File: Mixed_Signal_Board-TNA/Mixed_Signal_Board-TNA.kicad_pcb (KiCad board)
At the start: 4 copper layers, 109 parts, among them J200 USB_C_Receptacle_USB2.0_14P, J201 2x5 1.27mm, J300 031-5640-1010, J400 031-5640-1010, U100 HT7533, U102 TLV62569DBV, U2 MCP6001T-E/OT, U200 STM32F103CBT6, U201 USBLC6-2SC6, U300 MCP6001T-E/OT, U301 MCP6001T-E/OT, U302 REF3033AIDBZT, U303 ADC141S626CIMM_NOPB, U304 MCP6001T-E/OT, U400 DAC7563SDGSR, Y200 16MHz

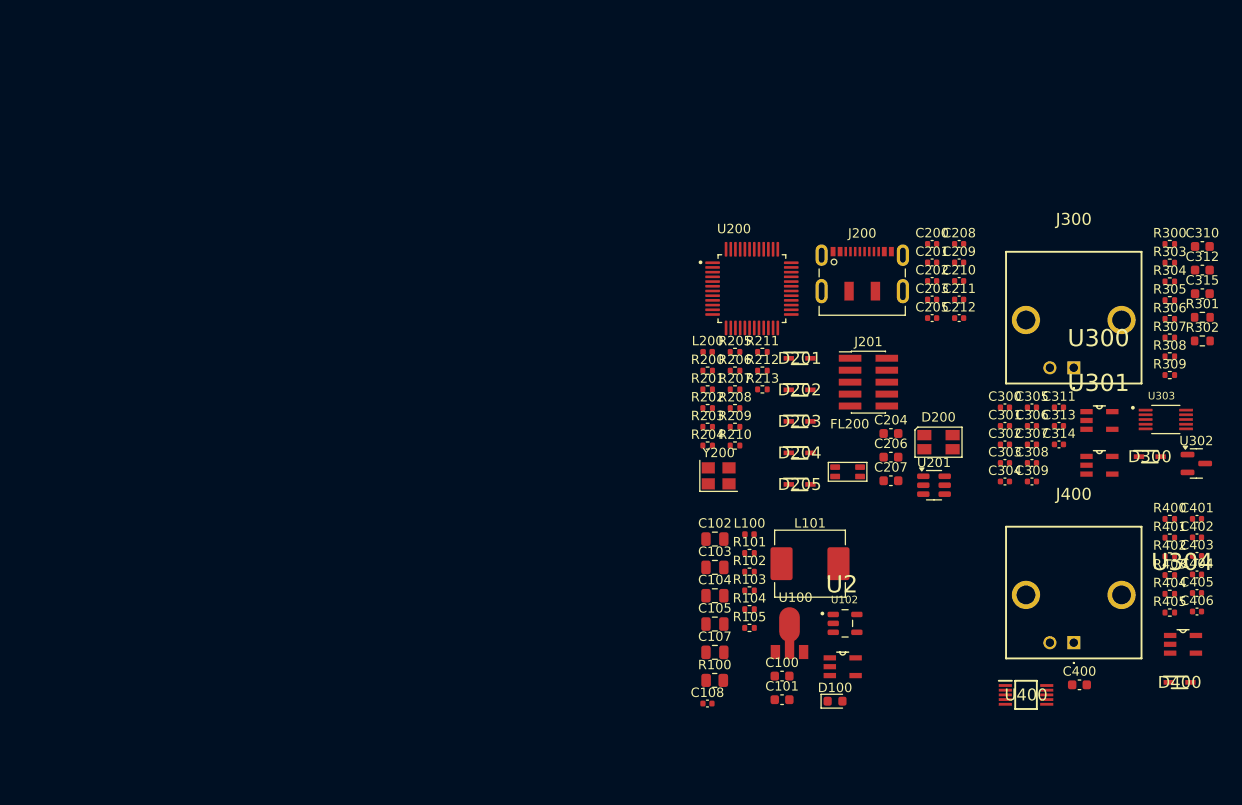
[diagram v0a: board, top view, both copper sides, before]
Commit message: Done Layout
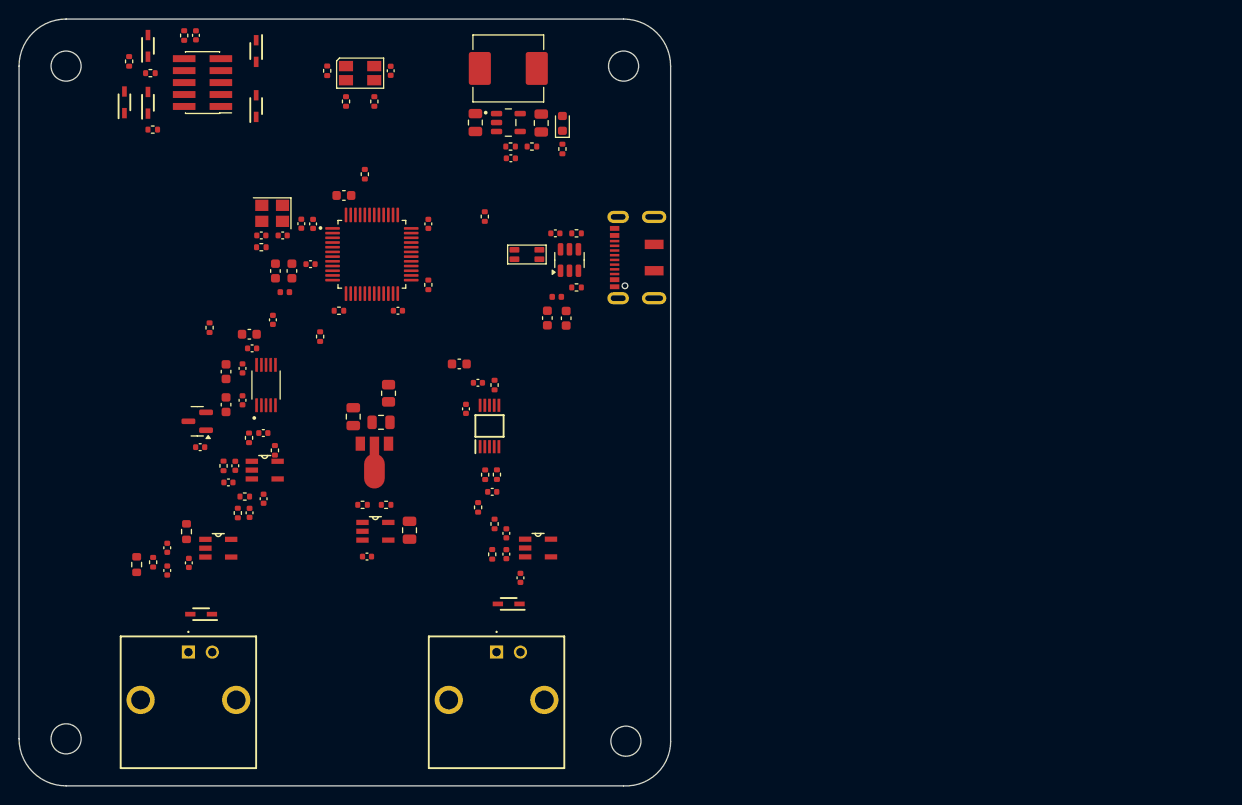
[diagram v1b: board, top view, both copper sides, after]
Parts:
- added C106: DNP, Capacitor_SMD:C_0402_1005Metric, F.Cu at (145.0, 58.5)
- added H1: MountingHole, MountingHole:MountingHole_3.2mm_M3, F.Cu at (97.8, 120.2)
- added H2: MountingHole, MountingHole:MountingHole_3.2mm_M3, F.Cu at (157.2, 120.5)
- added H3: MountingHole, MountingHole:MountingHole_3.2mm_M3, F.Cu at (97.8, 48.8)
- added H4: MountingHole, MountingHole:MountingHole_3.2mm_M3, F.Cu at (157.0, 48.8)
- moved R301 116.3 mm to (105.2, 101.7), turned to 90 degrees
- moved R300 113.2 mm to (107.0, 101.5), turned to -90 degrees
- moved R302 109.9 mm to (110.5, 98.2), turned to 90 degrees
- moved U302 106.3 mm to (111.7, 86.5), turned to 180 degrees
- moved C310 105.1 mm to (114.8, 84.7), turned to 90 degrees
- moved C312 104.3 mm to (114.8, 81.2), turned to -90 degrees
- moved R303 102.6 mm to (116.0, 96.2), turned to -90 degrees
- moved D300 102.2 mm to (112.1, 107.0), turned to 180 degrees
- moved R305 102.1 mm to (114.5, 91.2), turned to -90 degrees
- moved R308 102.1 mm to (113.0, 76.5), turned to 90 degrees
- moved C315 101.4 mm to (117.2, 77.2), turned to 180 degrees
- moved R304 100.9 mm to (116.7, 94.5)
- moved J300 98.8 mm to (110.8, 111.0), turned to 180 degrees
- moved R307 98.4 mm to (117.2, 88.3), turned to -90 degrees
- moved R306 96.1 mm to (119.9, 89.6), turned to -90 degrees
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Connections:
- net Net-(D200-BK) renamed /MCU/B
- net Net-(D200-GK) renamed /MCU/G
- net Net-(D200-RK) renamed /MCU/R
- net Net-(D202-K1) renamed /MCU/CONN_SWDIO
- net Net-(D203-K1) renamed /MCU/CONN_SWCLK
- net Net-(D204-K1) renamed /MCU/CONN_SWO
- net Net-(D205-K1) renamed /MCU/CONN_NRST
- C200 pad 2: <NO NET> -> VREF_DAC
- C201 pad 2: <NO NET> -> VREF_DAC
- C202 pad 2: <NO NET> -> VREF_DAC
- C203 pad 2: <NO NET> -> VREF_DAC
- C204 pad 2: <NO NET> -> VREF_DAC
- C205 pad 2: <NO NET> -> VREF_DAC
- C206 pad 2: <NO NET> -> VREF_DAC
- C207 pad 2: <NO NET> -> VREF_DAC
- C208 pad 2: <NO NET> -> VREF_DAC
- C209 pad 2: <NO NET> -> VREF_DAC
- C210 pad 2: <NO NET> -> VREF_DAC
- C211 pad 1: <NO NET> -> VREF_DAC
- C212 pad 1: <NO NET> -> VREF_DAC
- D201 pad 2: <NO NET> -> VREF_DAC
- D202 pad 2: <NO NET> -> VREF_DAC
- D203 pad 2: <NO NET> -> VREF_DAC
- D204 pad 2: <NO NET> -> VREF_DAC
- D205 pad 2: <NO NET> -> VREF_DAC
- J200 pad A1: <NO NET> -> VREF_DAC
- J200 pad A12: <NO NET> -> VREF_DAC
- J200 pad B1: <NO NET> -> VREF_DAC
- J200 pad B12: <NO NET> -> VREF_DAC
- J201 pad 3: <NO NET> -> VREF_DAC
- J201 pad 5: <NO NET> -> VREF_DAC
- J201 pad 9: <NO NET> -> VREF_DAC
- R200 pad 1: <NO NET> -> VREF_DAC
- R205 pad 1: <NO NET> -> VREF_DAC
- R206 pad 1: <NO NET> -> VREF_DAC
- U200 pad 23: <NO NET> -> VREF_DAC
- U200 pad 35: <NO NET> -> VREF_DAC
- U200 pad 47: <NO NET> -> VREF_DAC
- U200 pad 8: <NO NET> -> VREF_DAC
- U201 pad 2: <NO NET> -> VREF_DAC
- Y200 pad 2: <NO NET> -> VREF_DAC
- Y200 pad 4: <NO NET> -> VREF_DAC
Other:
- board outline added: 69.3 x 81.5 mm
